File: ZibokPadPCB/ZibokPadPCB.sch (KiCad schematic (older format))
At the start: 68 parts, among them Q1 DTC123J, SW1 Rotary_Encoder_Switch, U1 STM32F072C8Tx, U2 USBLC6-2SC6, U3 MCP1700-3302E_SOT23

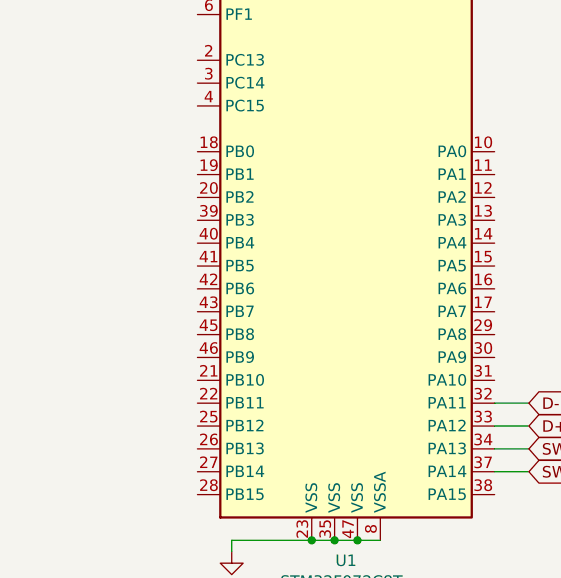
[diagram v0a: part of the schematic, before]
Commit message: Routing
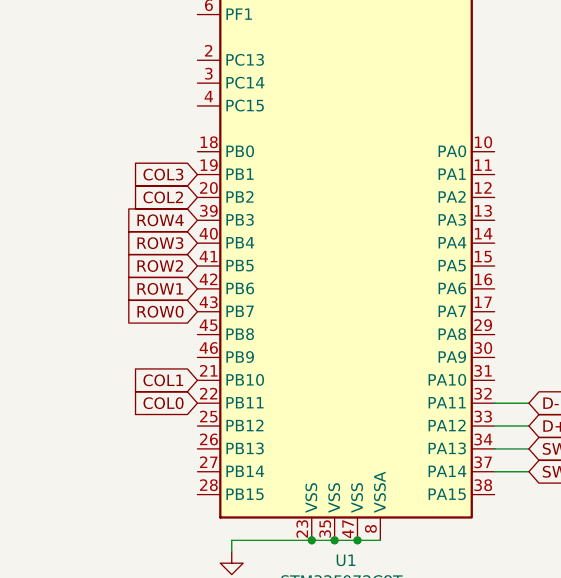
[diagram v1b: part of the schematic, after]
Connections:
- net COL0: now also U1.22 (PB11)
- net COL1: now also U1.21 (PB10)
- net COL2: now also U1.20 (PB2)
- net COL3: now also U1.19 (PB1)
- net ROW0: now also U1.43 (PB7)
- net ROW1: now also U1.42 (PB6)
- net ROW2: now also U1.41 (PB5)
- net ROW3: now also U1.40 (PB4)
- net ROW4: now also U1.39 (PB3)
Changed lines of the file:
@@
 Wire Wire Line
 	950  600  1150 600
+Text GLabel 1350 5100 0    50   Input ~ 0
+ROW0
+Text GLabel 1350 5000 0    50   Input ~ 0
+ROW1
+Text GLabel 1350 4900 0    50   Input ~ 0
+ROW2
+Text GLabel 1350 4800 0    50   Input ~ 0
+ROW3
+Text GLabel 1350 4700 0    50   Input ~ 0
+ROW4
+Text GLabel 1350 5500 0    50   Input ~ 0
+COL0
+Text GLabel 1350 5400 0    50   Input ~ 0
+COL1
+Text GLabel 1350 4600 0    50   Input ~ 0
+COL2
+Text GLabel 1350 4500 0    50   Input ~ 0
+COL3
 $EndSCHEMATC
